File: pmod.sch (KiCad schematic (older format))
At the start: 12 parts, among them J4 PMOD, U4 LP2985-3.3, U5 TXS0108EPW

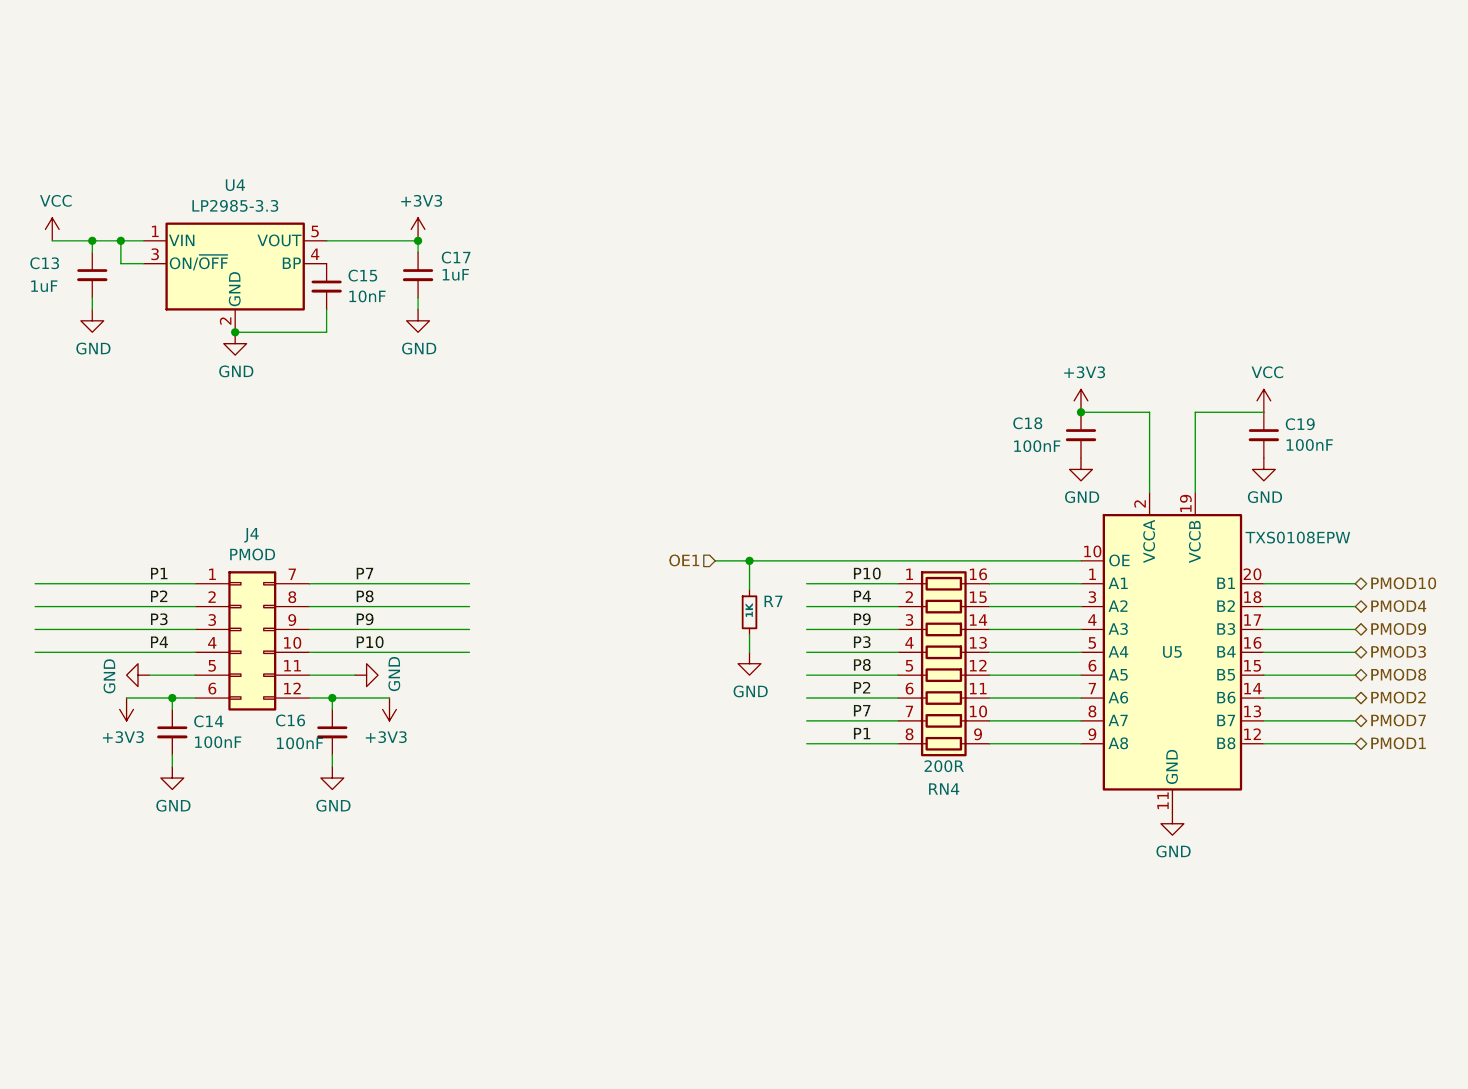
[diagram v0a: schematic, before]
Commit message: do over with additional pmod
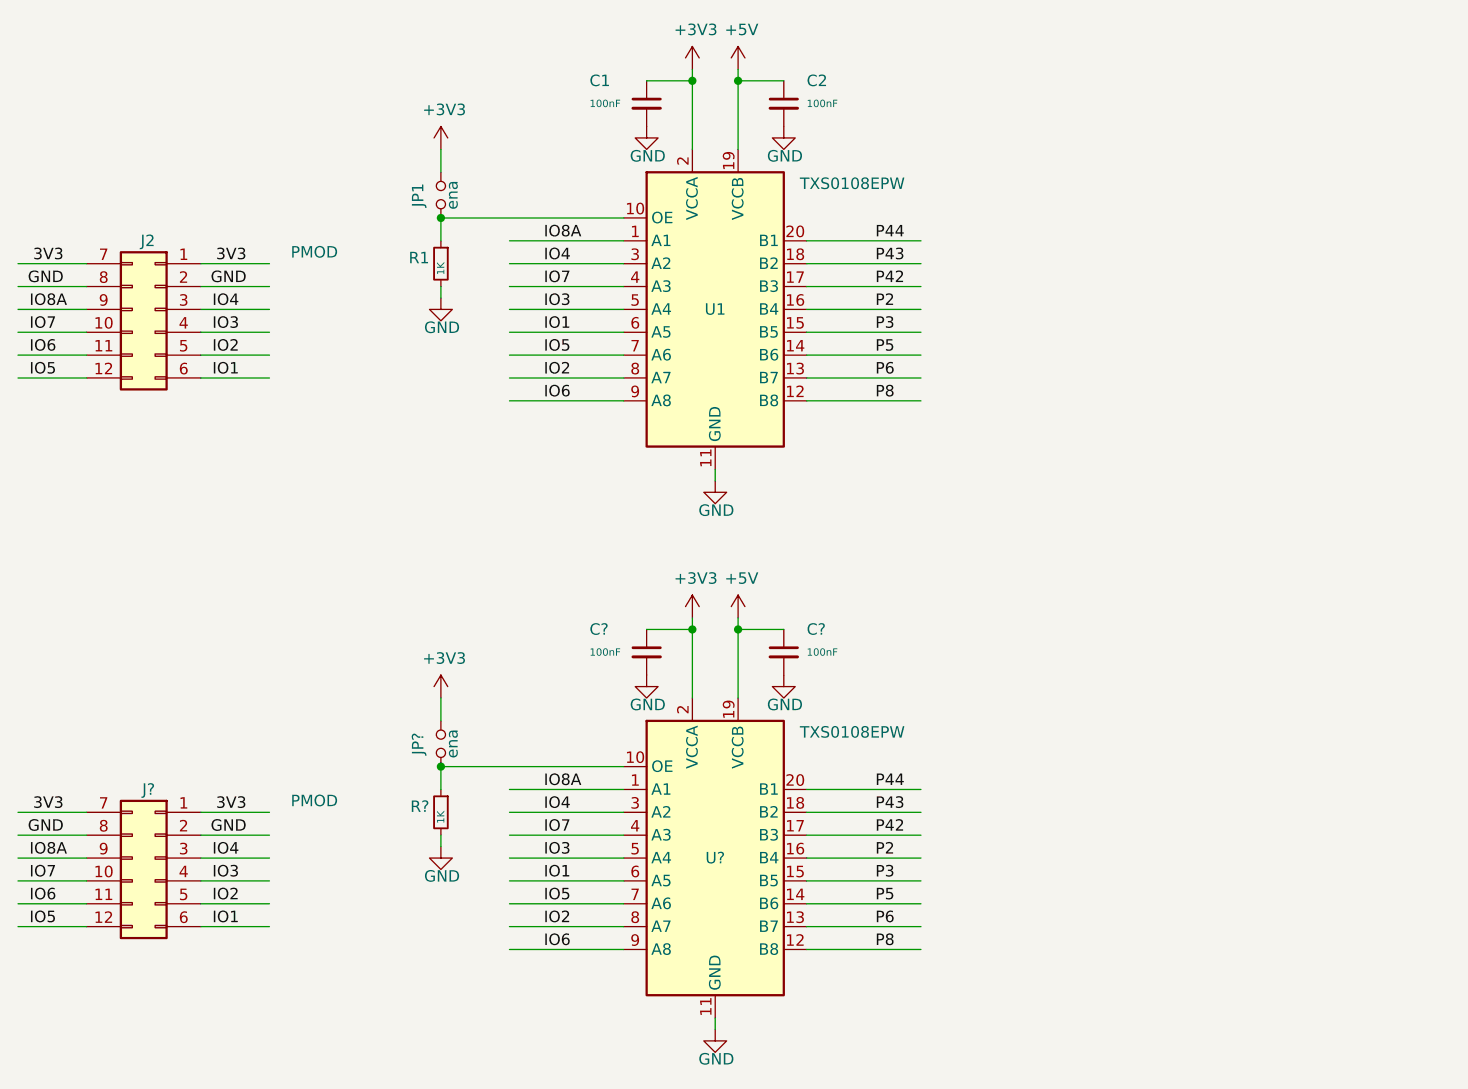
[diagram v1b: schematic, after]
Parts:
- removed C13, C17: 1uF, Capacitor_SMD:C_0603_1608Metric_Pad1.05x0.95mm_HandSolder, symbol Device:C_Small
- removed C14, C16, C18, C19: 100nF, Capacitor_SMD:C_0603_1608Metric_Pad1.05x0.95mm_HandSolder, symbol Device:C_Small
- removed C15: 10nF, Capacitor_SMD:C_0603_1608Metric_Pad1.05x0.95mm_HandSolder, symbol Device:C_Small
- removed J4: PMOD, Connector_PinSocket_2.54mm:PinSocket_2x06_P2.54mm_Horizontal_Top_Bottom, symbol Connector_Generic:Conn_02x06_Top_Bottom
- removed R7: 1K, Resistor_SMD:R_0603_1608Metric_Pad1.05x0.95mm_HandSolder, symbol Device:R_Small
- removed RN4: 200R, Resistor_SMD:R_Cat16-8, symbol Device:R_Pack08
- removed U4: LP2985-3.3, Package_TO_SOT_SMD:SOT-23-5, symbol Regulator_Linear:LP2985-3.3
- removed U5: TXS0108EPW, Package_SO:TSSOP-20_4.4x6.5mm_P0.65mm, symbol Logic_LevelTranslator:TXS0108EPW
- added C1, C2, C? (x2): 100nF, Capacitor_SMD:C_0603_1608Metric_Pad1.05x0.95mm_HandSolder, symbol Device:C_Small
- added J2, J?: PMOD, max_breakout:PinSocket_2x06_Top_Bottom_P2.54mm_Horizontal, symbol Connector_Generic:Conn_02x06_Top_Bottom
- added JP1, JP?: ena, Connector_PinHeader_2.54mm:PinHeader_1x02_P2.54mm_Vertical, symbol Device:Jumper_NO_Small
- added R1, R?: 1K, Resistor_SMD:R_0603_1608Metric_Pad1.05x0.95mm_HandSolder, symbol Device:R_Small
- added U1, U?: TXS0108EPW, Package_SO:TSSOP-20_4.4x6.5mm_P0.65mm, symbol Logic_LevelTranslator:TXS0108EPW
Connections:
- net labels added: +5V, 3V3, IO1, IO2, IO3, IO4, IO5, IO6, IO7, IO8A, P42, P43, P44, P5, P6
- net labels removed: OE1, P1, P10, P4, P7, P9, PMOD1, PMOD10, PMOD2, PMOD3, PMOD4, PMOD7, PMOD8, PMOD9, VCC
- wire segments 62 -> 78
